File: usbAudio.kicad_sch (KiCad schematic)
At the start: 35 parts, among them J2 USB_C_Receptacle_USB2.0_14P, J3 AudioJack3, SW1 PLAY/PAUSE, SW2 NEXT TR., SW3 MUTE, SW4 VOL+, SW5 VOL-, SW6 PREV. TR., SW7 STOP, SW8 SW_SPDT, U1 PCM2706CPJTR, Y1 12MHz

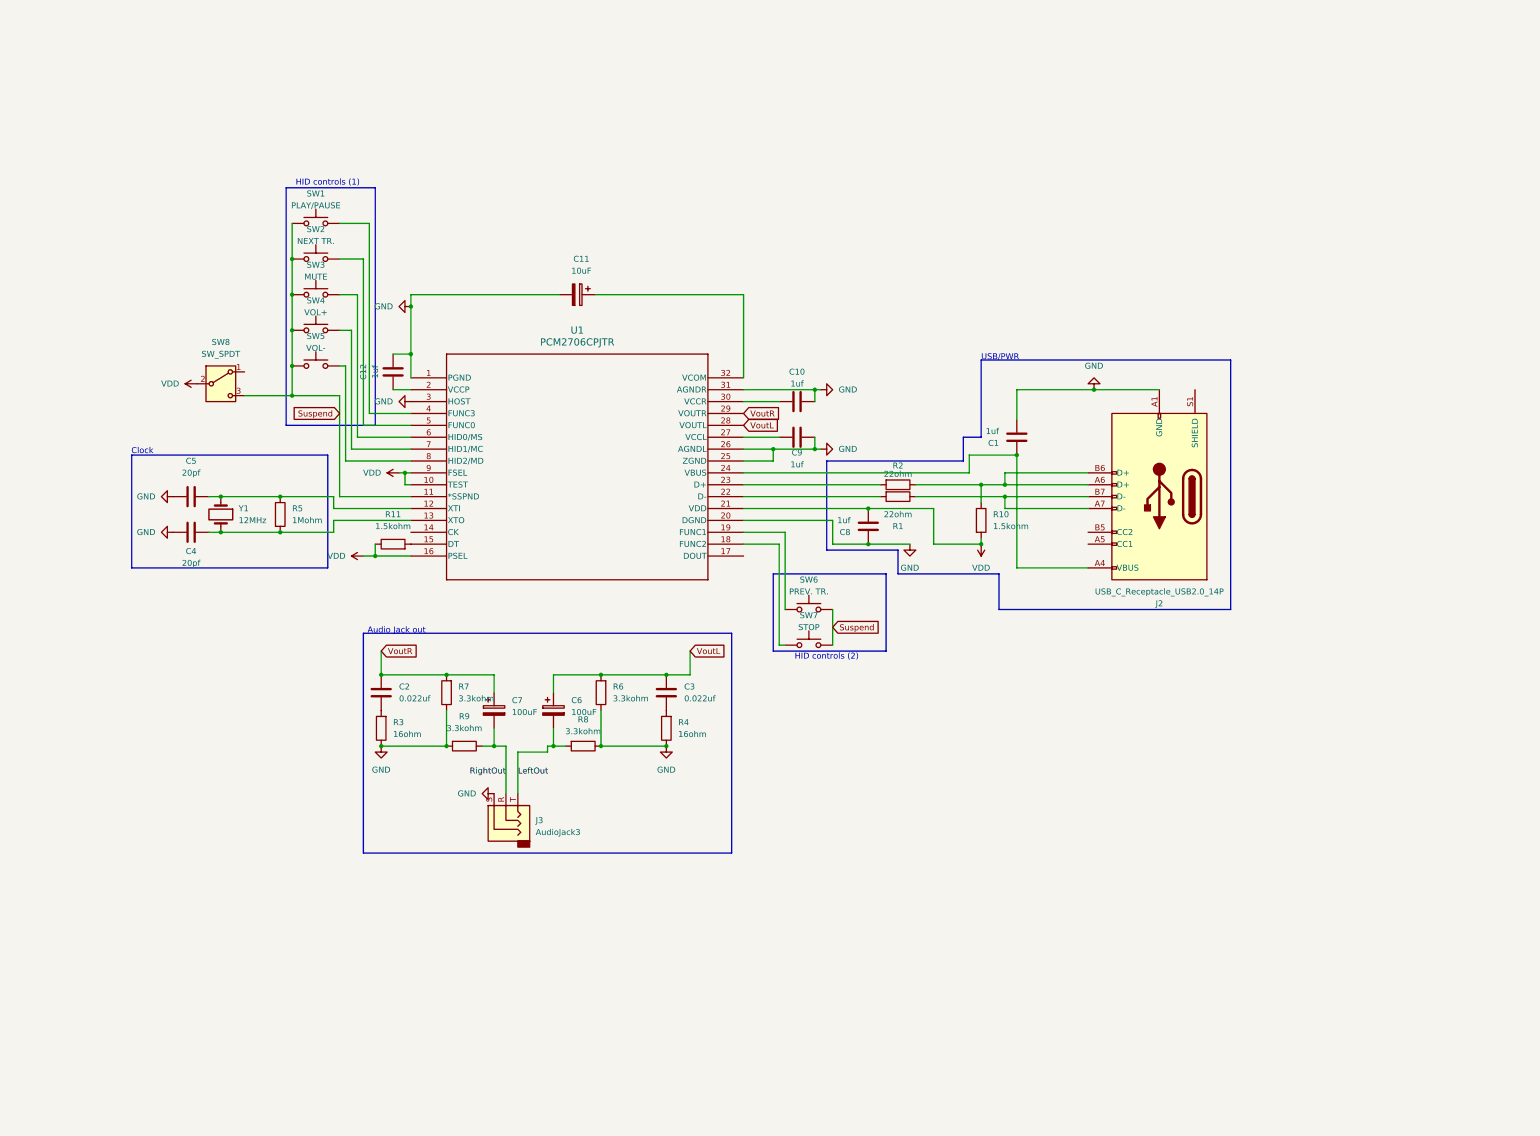
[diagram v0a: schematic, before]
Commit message: Start work on power side
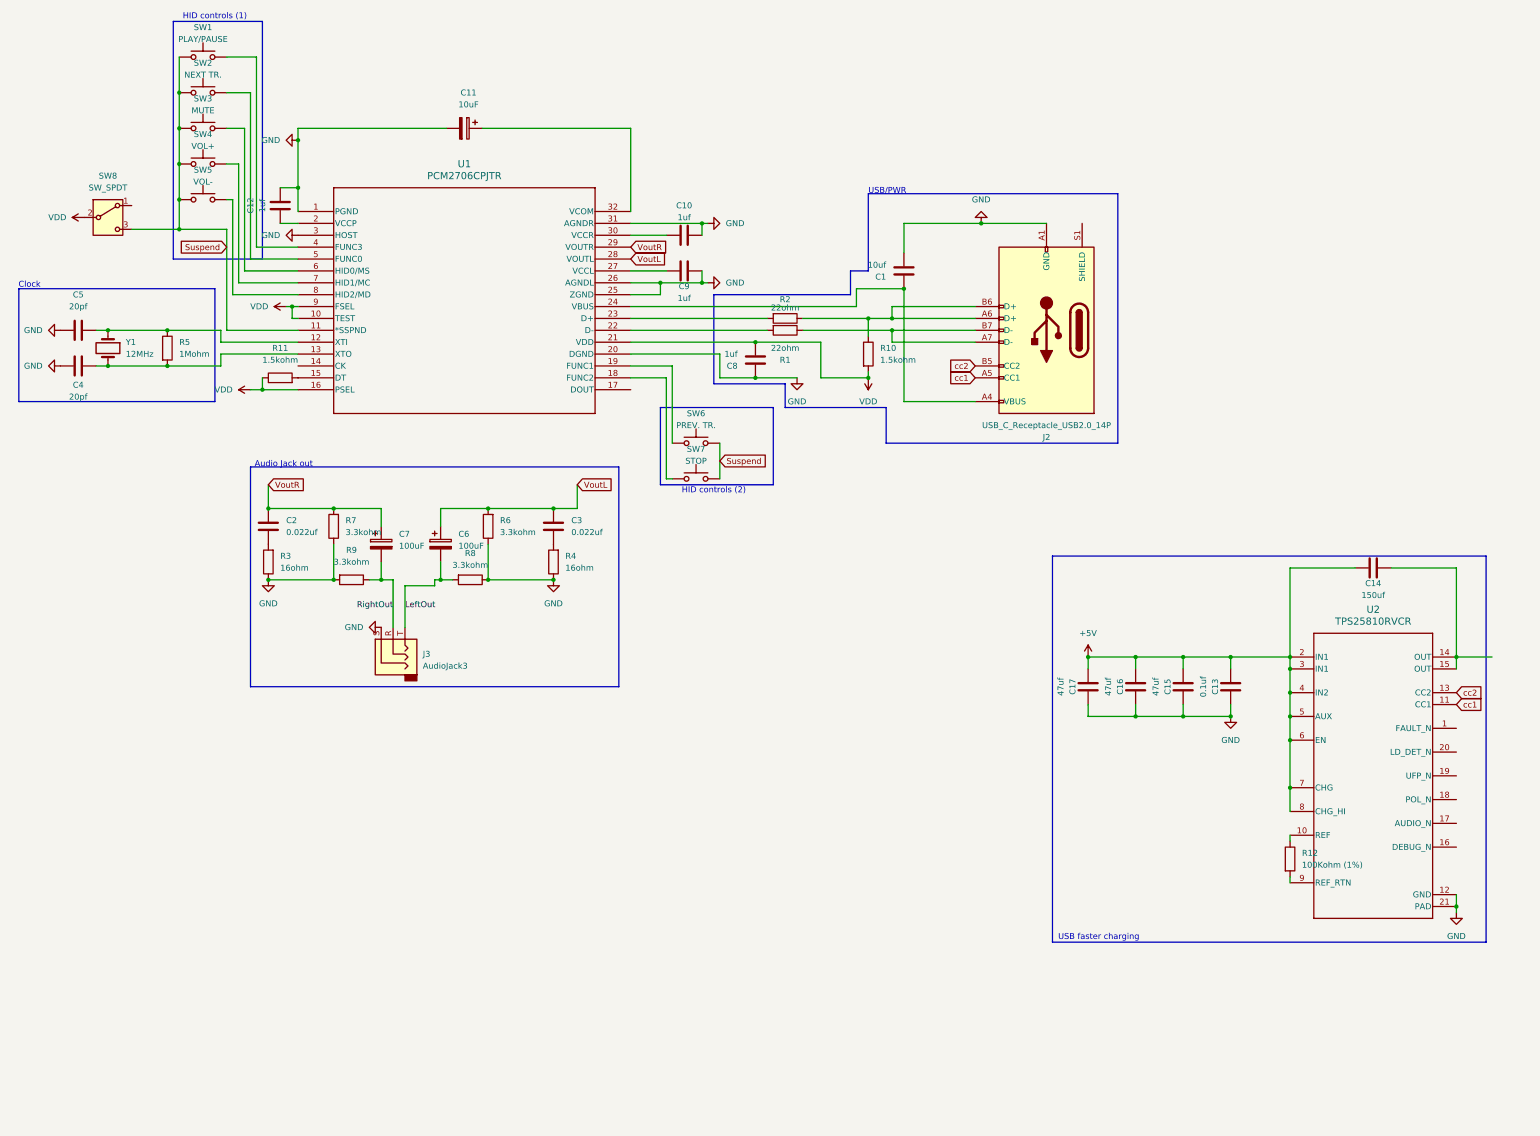
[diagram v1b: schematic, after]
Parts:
- added C13: 0.1uf, symbol Device:C
- added C14: 150uf, symbol Device:C
- added C15, C16, C17: 47uf, symbol Device:C
- added R12: 100Kohm (1%), symbol Device:R
- added U2: TPS25810RVCR, RVC0020A, symbol TPS25810:TPS25810RVCR
- C1: value 1uf -> 10uf
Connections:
- net GND: now also C13.2, C15.2, C16.2, C17.2, U2.12 (GND), U2.21 (PAD)
- net cc1: now reaches J2.A5 (CC1)
- net cc1: now also U2.11 (CC1)
- net cc2: now reaches J2.B5 (CC2)
- net cc2: now also U2.13 (CC2)
- new net: R12.1, U2.10 (REF)
- new net: R12.2, U2.9 (REF_RTN)
- new net: C14.2, U2.14 (OUT), U2.15 (OUT)
- new net +5V: C13.1, C14.1, C15.1, C16.1, C17.1, U2.2 (IN1), U2.3 (IN1), U2.4 (IN2), U2.5 (AUX), U2.6 (EN), U2.7 (CHG), U2.8 (CHG_HI)
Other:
- note added: "USB faster charging"
- moved on the sheet: C1, C10, C11, C12, C2, C3, C4, C5, C6, C7, C8, C9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

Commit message: Finish schem!
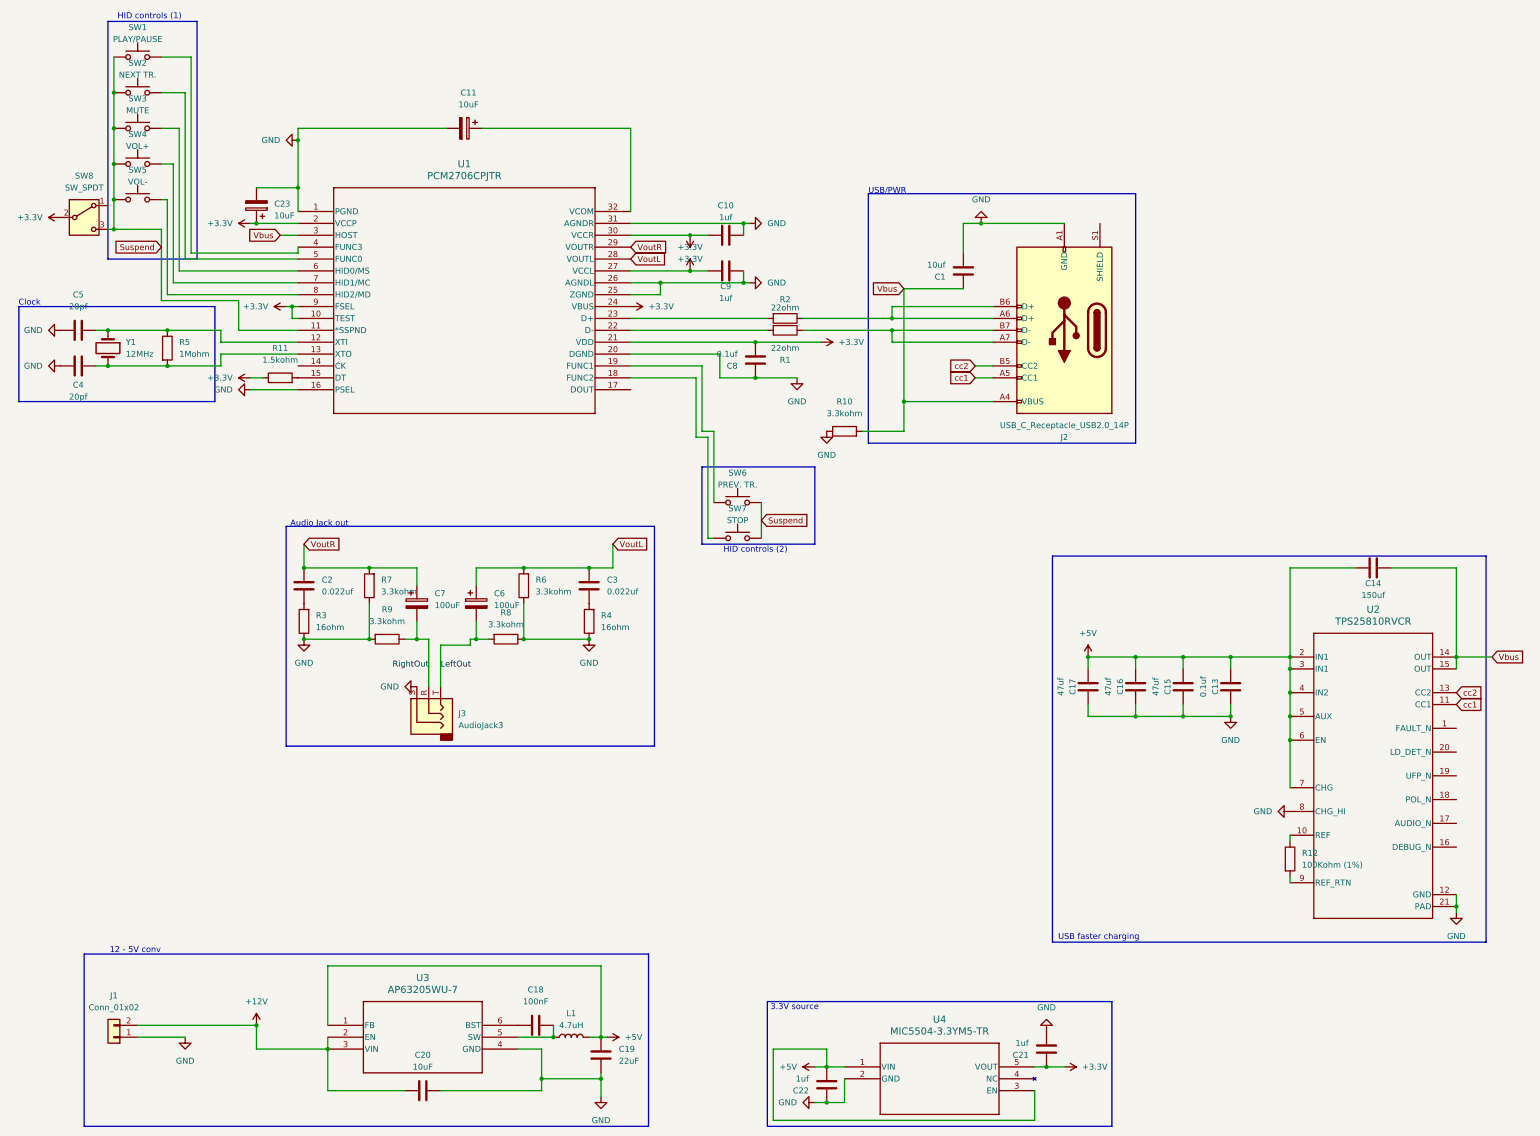
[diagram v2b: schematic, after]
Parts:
- removed C12: 1uf, symbol Device:C
- added C18: 100nF, symbol Device:C
- added C19: 22uF, symbol Device:C
- added C20: 10uF, symbol Device:C
- added C21, C22: 1uf, symbol Device:C
- added C23: 10uF, symbol Device:C_Polarized
- added J1: Conn_01x02, symbol Connector_Generic:Conn_01x02
- added L1: 4.7uH, symbol Device:L
- added U3: AP63205WU-7, AP63205:SOIC_05WU-7_DIO, symbol AP63205:AP63205WU-7
- added U4: MIC5504-3.3YM5-TR, SOT-23-5_MC_MCH, symbol MIC5504-3.3YM5:MIC5504-3.3YM5-TR
- C8: value 1uf -> 0.1uf
- R10: value 1.5kohm -> 3.3kohm
- U1: footprint PJT32 -> (none)
- U2: footprint RVC0020A -> TPS25810:RVC0020A
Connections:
- net +5V: now also C19.2, C22.1, L1.2, U3.1 (FB), U4.1 (VIN), U4.3 (EN); no longer U2.8 (CHG_HI)
- net GND: now also R10.1, U1.16 (PSEL), U2.8 (CHG_HI), C19.1, C20.1, C21.1, C22.2, C23.2, J1.1 (Pin_1), U3.4 (GND), U4.2 (GND); no longer U1.3 (HOST)
- net +3.3V: now reaches U1.2 (VCCP)
- net +3.3V: now also C10.1, C8.1, C9.1, R11.1, SW8.2 (B), U1.10 (TEST), U1.21 (VDD), U1.24 (VBUS), U1.27 (VCCL), U1.30 (VCCR), U1.9 (FSEL), C21.2, C23.1, U4.5 (VOUT)
- net Vbus: now reaches C1.2, J2.A4 (VBUS), J2.A9 (VBUS), J2.B4 (VBUS), J2.B9 (VBUS)
- net Vbus: now also C14.2, R10.2, U1.3 (HOST), U2.14 (OUT), U2.15 (OUT); no longer U1.24 (VBUS)
- net at J2.A6 (D+), J2.B6 (D+), R2.1: no longer R10.1
- removed net VDD: C8.1, R10.2, R11.1, SW8.2 (B), U1.10 (TEST), U1.16 (PSEL), U1.21 (VDD), U1.9 (FSEL)
- new net: C18.2, L1.1, U3.5 (SW)
- new net: C18.1, U3.6 (BST)
- new net +12V: C20.2, J1.2 (Pin_2), U3.2 (EN), U3.3 (VIN)
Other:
- note added: "12 - 5V conv"
- note added: "3.3V source"
- moved on the sheet: C1, C10, C2, C3, C6, C7, C9, J2, J3, R3, R4, R6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
